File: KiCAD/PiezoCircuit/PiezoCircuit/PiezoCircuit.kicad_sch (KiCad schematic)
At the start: 14 parts, among them U1 ${SIM.PARAMS}, U2 ${SIM.PARAMS}

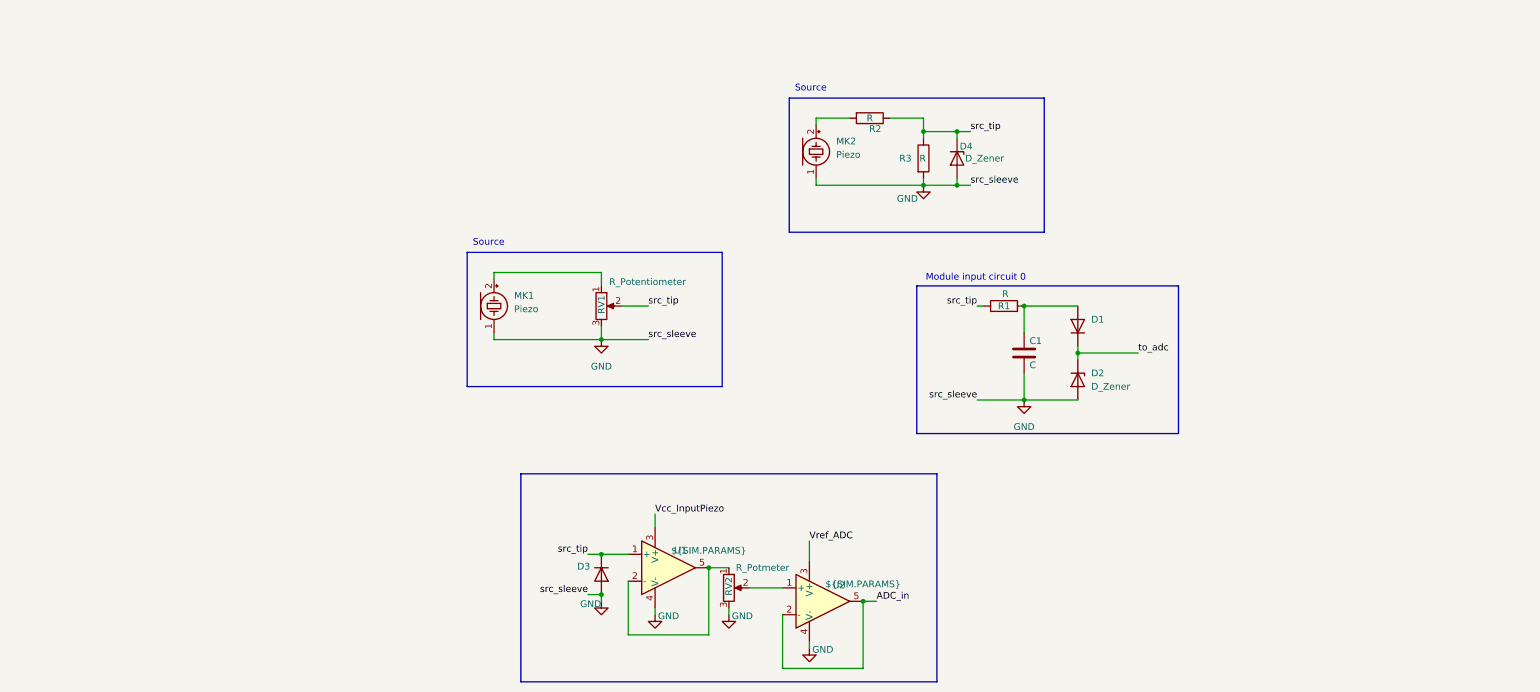
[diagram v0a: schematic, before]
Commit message: Create InstrumentApp
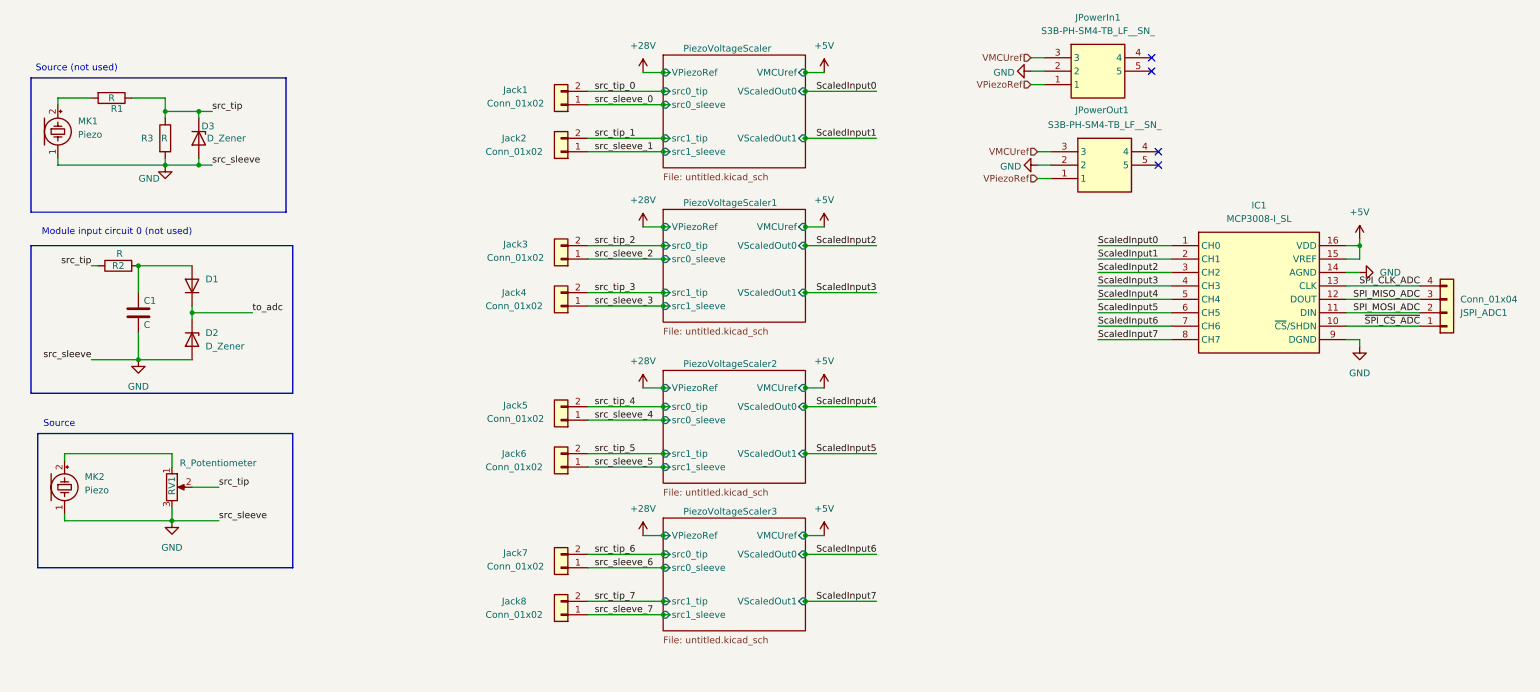
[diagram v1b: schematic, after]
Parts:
- removed D3: ~, Diode_THT:D_DO-41_SOD81_P10.16mm_Horizontal, symbol Diode:1N4001
- removed RV2: R_Potmeter, symbol Device:R_Potentiometer
- removed U1, U2: ${SIM.PARAMS}, symbol Simulation_SPICE:OPAMP
- added IC1: MCP3008-I_SL, SOIC127P600X175-16N, symbol MCP3008-I_SL:MCP3008-I_SL
- added JPowerIn1, JPowerOut1: S3B-PH-SM4-TB_LF__SN_, S3BPHSM4TBLFSN, symbol S3B-PH-SM4-TB_LF__SN_:S3B-PH-SM4-TB_LF__SN_
- added JSPI_ADC1: Conn_01x04, Connector_JST:JST_PH_S4B-PH-SM4-TB_1x04-1MP_P2.00mm_Horizontal, symbol Connector_Generic:Conn_01x04
- added Jack1, Jack2, Jack3, Jack4, Jack5, Jack6, Jack7, Jack8: Conn_01x02, Connector_JST:JST_PH_S2B-PH-SM4-TB_1x02-1MP_P2.00mm_Horizontal, symbol Connector_Generic:Conn_01x02
- D1: value ~ -> (none)
- renumbered D4 to D3, MK2 to MK1, MK1 to MK2, R2 to R1, R1 to R2
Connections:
- net GND: now also IC1.14 (AGND), IC1.9 (DGND), JPowerIn1.2, JPowerOut1.2
- new net +5V: IC1.15 (VREF), IC1.16 (VDD)
- new net SPI_CLK_ADC: IC1.13 (CLK), JSPI_ADC1.4 (Pin_4)
- new net SPI_MISO_ADC: IC1.12 (DOUT), JSPI_ADC1.3 (Pin_3)
- new net SPI_MOSI_ADC: IC1.11 (DIN), JSPI_ADC1.2 (Pin_2)
- new net ScaledInput0: IC1.1 (CH0)
- new net ScaledInput1: IC1.2 (CH1)
- new net ScaledInput2: IC1.3 (CH2)
- new net ScaledInput3: IC1.4 (CH3)
- new net ScaledInput4: IC1.5 (CH4)
- new net ScaledInput5: IC1.6 (CH5)
- new net ScaledInput6: IC1.7 (CH6)
- new net ScaledInput7: IC1.8 (CH7)
- new net VMCUref: JPowerIn1.3, JPowerOut1.3
- new net VPiezoRef: JPowerIn1.1, JPowerOut1.1
- new net src_sleeve_0: Jack1.1 (Pin_1)
- new net src_sleeve_1: Jack2.1 (Pin_1)
- new net src_sleeve_2: Jack3.1 (Pin_1)
- new net src_sleeve_3: Jack4.1 (Pin_1)
- new net src_sleeve_4: Jack5.1 (Pin_1)
- new net src_sleeve_5: Jack6.1 (Pin_1)
- new net src_sleeve_6: Jack7.1 (Pin_1)
- new net src_sleeve_7: Jack8.1 (Pin_1)
- new net src_tip_0: Jack1.2 (Pin_2)
- new net src_tip_1: Jack2.2 (Pin_2)
- new net src_tip_2: Jack3.2 (Pin_2)
- new net src_tip_3: Jack4.2 (Pin_2)
- new net src_tip_4: Jack5.2 (Pin_2)
- new net src_tip_5: Jack6.2 (Pin_2)
- new net src_tip_6: Jack7.2 (Pin_2)
- new net src_tip_7: Jack8.2 (Pin_2)
- new net ~{SPI_CS_ADC}: IC1.10 (~{CS}/SHDN), JSPI_ADC1.1 (Pin_1)
- no-connect marks 0 -> 4
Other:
- added sheet PiezoVoltageScaler (untitled.kicad_sch)
- added sheet PiezoVoltageScaler1 (untitled.kicad_sch)
- added sheet PiezoVoltageScaler2 (untitled.kicad_sch)
- added sheet PiezoVoltageScaler3 (untitled.kicad_sch)
- note added: "Module input circuit 0 (not used)"
- note added: "Source (not used)"
- note removed: "Module input circuit 0"
- moved on the sheet: C1, D1, D2, D3, MK1, MK2, R1, R2, R3, RV1
